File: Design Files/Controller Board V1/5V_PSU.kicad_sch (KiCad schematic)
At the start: 9 parts, among them IC1 LMR66410MC5RXBRQ1

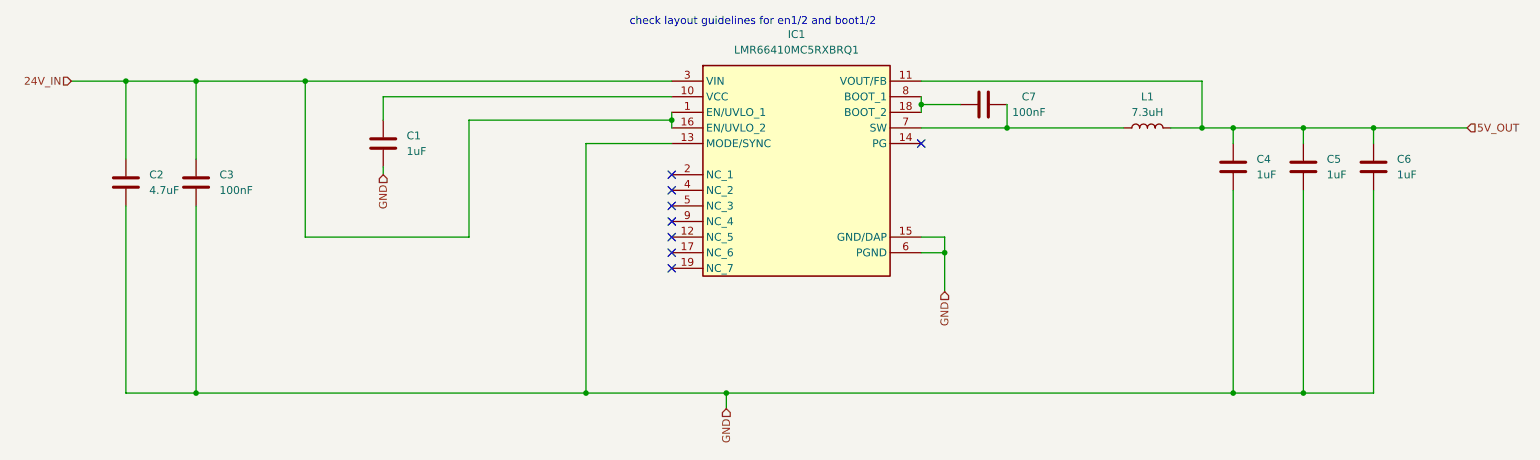
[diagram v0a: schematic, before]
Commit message: Made the THING
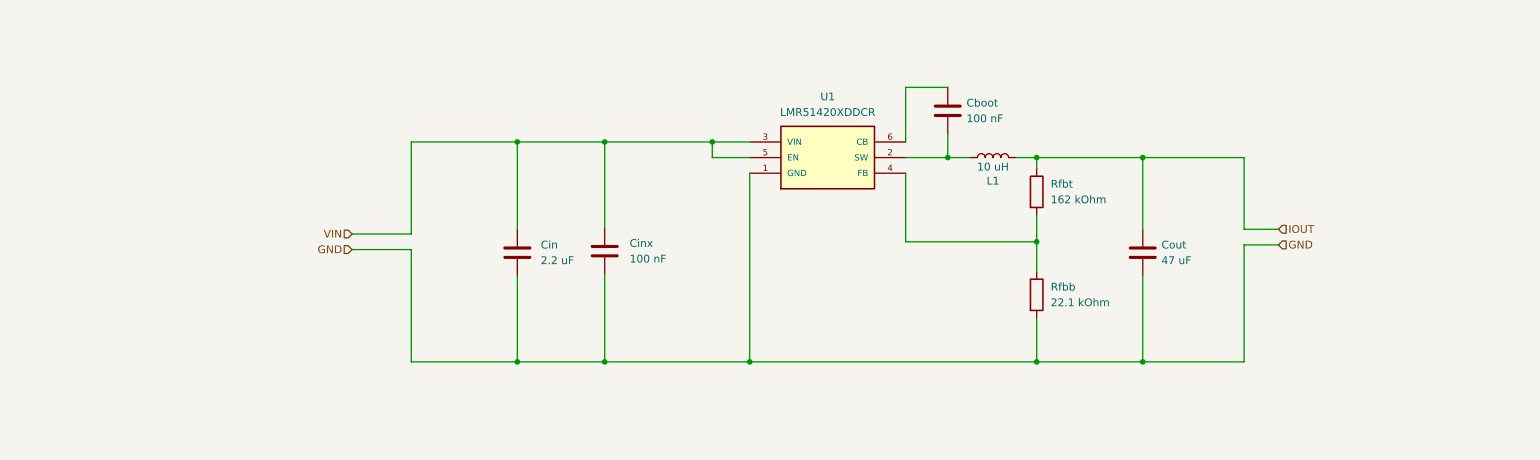
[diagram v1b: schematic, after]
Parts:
- removed C1, C4, C5, C6: 1uF, symbol Device:C
- removed C2: 4.7uF, symbol Device:C
- removed C3, C7: 100nF, symbol Device:C
- removed IC1: LMR66410MC5RXBRQ1, LMR66430R5RXBR, symbol LMR66410MC5RXBRQ1:LMR66410MC5RXBRQ1
- added Cboot: 100 nF, Capacitor_SMD:C_0402_1005Metric_Pad0.74x0.62mm_HandSolder, symbol Device:C
- added Cin: 2.2 uF, Capacitor_SMD:C_1206_3216Metric_Pad1.33x1.80mm_HandSolder, symbol Device:C
- added Cinx: 100 nF, Capacitor_SMD:C_0603_1608Metric_Pad1.08x0.95mm_HandSolder, symbol Device:C
- added Cout: 47 uF, Capacitor_SMD:C_1210_3225Metric_Pad1.33x2.70mm_HandSolder, symbol Device:C
- added Rfbb: 22.1 kOhm, Resistor_SMD:R_0402_1005Metric_Pad0.72x0.64mm_HandSolder, symbol Device:R
- added Rfbt: 162 kOhm, Resistor_SMD:R_0402_1005Metric_Pad0.72x0.64mm_HandSolder, symbol Device:R
- added U1: LMR51420XDDCR, LMR51420XDDCR:SOT95P280X110-6N, symbol LMR51420XDDCR:LMR51420XDDCR
- L1: value 7.3uH -> 10 uH; footprint (none) -> NRS8030T100MJGJ:IND_TAIYO_NRS8030_TAY
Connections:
- net GND: now also Cin.2, Cinx.2, Cout.2, Rfbb.2, U1.1 (GND)
- net at L1.1: now also Cboot.2, U1.2 (SW)
- net 5V_OUT renamed IOUT
- net IOUT: now also Cout.1, Rfbt.1
- new net: Rfbb.1, Rfbt.2, U1.4 (FB)
- new net: Cboot.1, U1.6 (CB)
- new net VIN: Cin.1, Cinx.1, U1.3 (VIN), U1.5 (EN)
- no-connect marks 8 -> 0
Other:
- note removed: "check layout guidelines for en1/2 and boot1/2"
